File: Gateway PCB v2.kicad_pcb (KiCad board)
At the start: 4 copper layers, 84.4 x 39.8 mm, 114 parts, among them J1 Conn_Coaxial, J2 Conn_01x04_Pin, J3 Conn_02x03_Odd_Even, J4 Conn_01x03_Pin, U6 TPS7A91, U7 TLV62568ADRL, X1 TG2016SMN 32.0000M-TCGNNMB

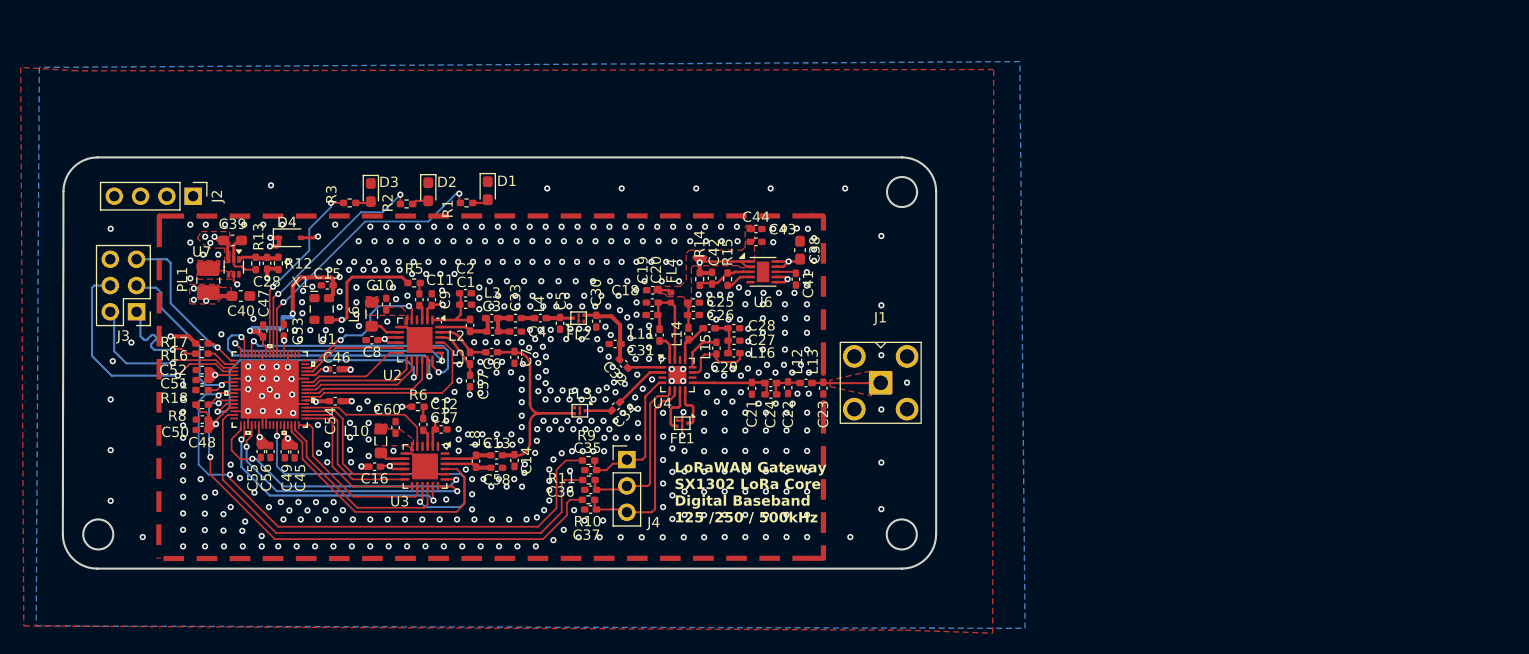
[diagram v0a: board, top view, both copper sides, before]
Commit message: Fail Save 3
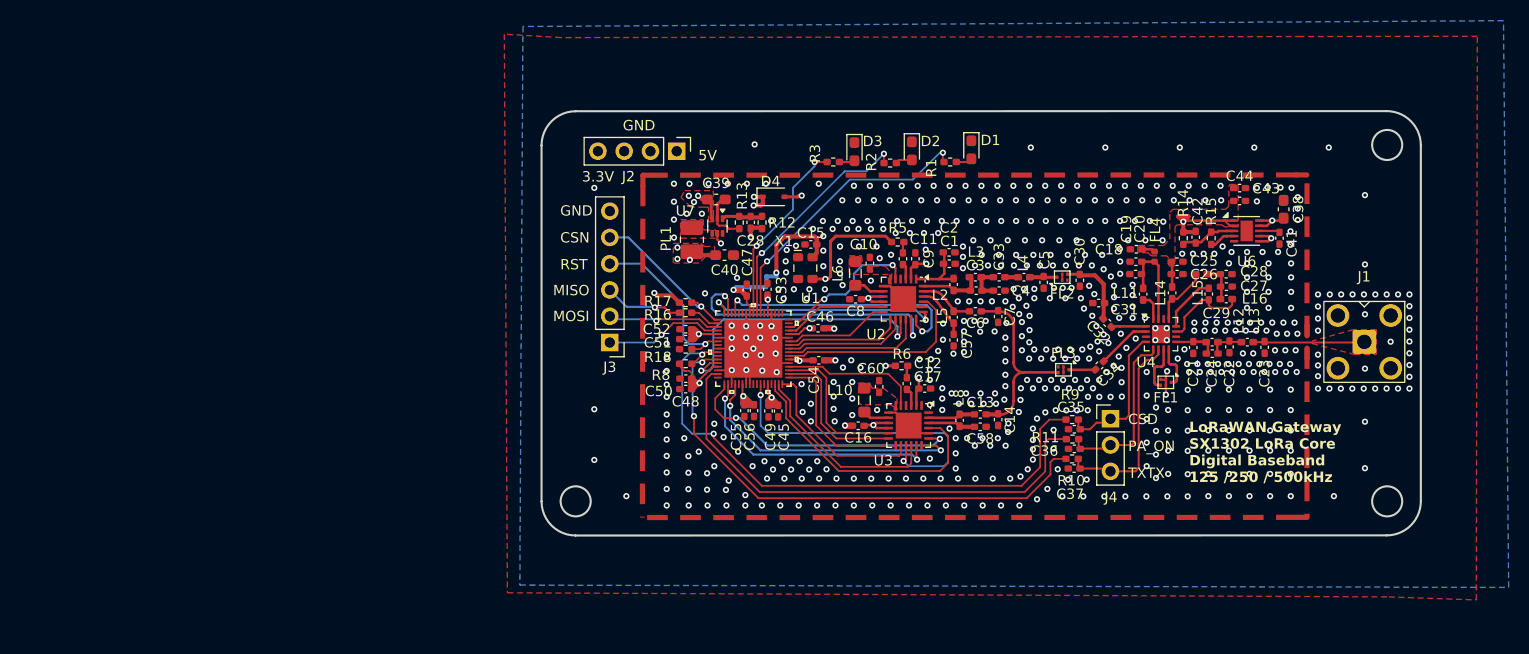
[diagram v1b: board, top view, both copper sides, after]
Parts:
- J3: footprint Connector_PinHeader_2.54mm:PinHeader_2x03_P2.54mm_Vertical -> Connector_PinHeader_2.54mm:PinHeader_1x06_P2.54mm_Vertical
- moved C27 47.9 mm to (125.5, 77.2)
- moved C28 47.9 mm to (125.4, 76.0)
- moved C29 47.9 mm to (123.8, 77.9)
- moved L15 47.9 mm to (123.0, 76.0)
- moved L16 47.9 mm to (125.4, 78.4)
- moved NT2 47.0 mm to (133.2, 83.6)
- moved J2 47.0 mm to (72.3, 64.1)
- moved C38 46.9 mm to (131.0, 69.7)
- moved C1 46.9 mm to (98.7, 75.0)
- moved C47 46.9 mm to (79.1, 77.5)
- moved C51 46.9 mm to (73.2, 82.3)
- moved C53 46.9 mm to (81.1, 77.4)
- moved C54 46.9 mm to (86.1, 84.3)
- moved C57 46.9 mm to (99.1, 82.4)
- moved L10 46.9 mm to (90.5, 88.2)
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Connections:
- J3 pad 1: EX_HOST_MISO -> EX_HOST_SCK
- J3 pad 3: EX_HOST_RESET -> EX_HOST_MISO
- J3 pad 4: EX_HOST_SCK -> EX_HOST_RESET
- J3 pad 6: unconnected-(J3-Pin_6-Pad6) -> GND
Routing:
- net EX_HOST_SCK: track 24.4 -> 11.9 mm
- net EX_HOST_MOSI: track 16.3 -> 11.0 mm
- net Net-(J1-In): track 7.01 -> 11.8 mm
- net Net-(U4-ANT): track 8.29 -> 4.19 mm
- net EX_HOST_MISO: track 10.2 -> 7.63 mm
- net GND2: track 5.83 -> 3.83 mm
- net Net-(U4-PA_OUT): track 3.97 -> 5.71 mm
- net EX_HOST_CSN: track 16.5 -> 14.8 mm
- net Net-(U4-TX_IN): track 7.42 -> 8.90 mm
- net GND: track 49.5 -> 50.8 mm, vias 564 -> 605
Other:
- board size 84.4 x 39.8 mm -> 85 x 41 mm
- board text added: "3.3V"
- board text added: "5V"
- board text added: "CSD"
- board text added: "CSN"
- board text added: "GND"
- board text added: "MISO"
- board text added: "MOSI"
- board text added: "PA_ON"
- board text added: "RST"
- board text added: "TXTX"
